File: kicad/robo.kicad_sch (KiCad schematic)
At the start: 46 parts, among them J10 KF2EDGR-2.54-2P, J11 KF7620-7.62-2P, J12 KF2EDGR-2.54-2P, J13 KF2EDGR-2.54-2P, J14 KF7620-7.62-2P, J15 PM254-2-12-Z-8.5, J16 PM254-2-09-Z-8.5, J8 KF2EDGR-2.54-4P, J9 KF2EDGR-2.54-3P, U16 74LVC1G17SE-7, U18 TPS70933DBVR, U19 74LVC1G17SE-7

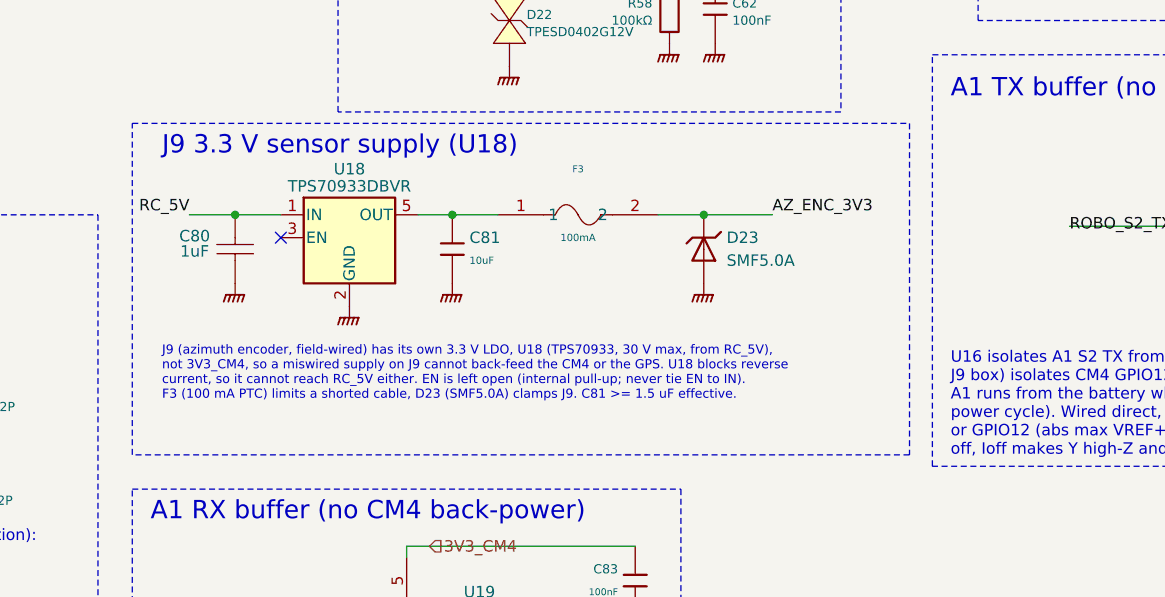
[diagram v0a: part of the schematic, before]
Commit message: Added notes
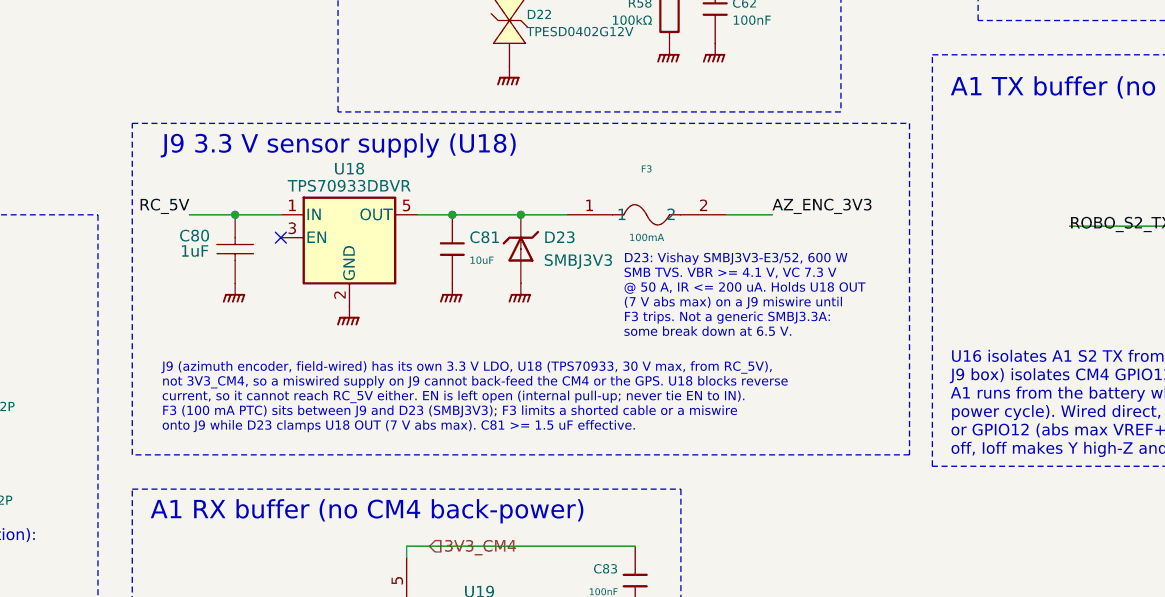
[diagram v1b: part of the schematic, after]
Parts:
- D23: value SMF5.0A -> SMBJ3V3; footprint MyPartsIPC:SODFL3718X110N -> MyPartsIPC:DIOM5436X244N; symbol MyParts:SMF5.0A -> MyParts:SMBJ3V3; LCSC Part C19077497 -> C82082; MPN SMF5.0A -> SMBJ3V3-E3/52; Manufacturer hongjiacheng -> Vishay; Pkg Type SMD SOD-123FL -> SMD SMB (DO-214AA)
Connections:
- net AZ_ENC_3V3: no longer D23.1
- net at C81.1, F3.1, U18.5 (OUT): now also D23.1
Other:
- note added: "D23: Vishay SMBJ3V3-E3/52, 600 W SMB TVS. VBR >= 4.1 V, VC 7.3 V @ 50 A, IR <= 200 uA. Holds U18 OUT (7 V abs max) on a J9 miswire until F3 trips. Not a generic SMBJ3.3A: some break down at 6.5 V."
- note added: "J9 (azimuth encoder, field-wired) has its own 3.3 V LDO, U18 (TPS70933, 30 V max, from RC_5V), not 3V3_CM4, so a miswired supply on J9 cannot back-feed the CM4 or the GPS. U18 blocks reverse current, so it cannot reach RC_5V either. EN is left open (internal pull-up; never tie EN to IN). F3 (100 mA PTC) sits between J9 and D23 (SMBJ3V3); F3 limits a shorted cable or a miswire onto J9 while D23 cl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"
- note removed: "J9 (azimuth encoder, field-wired) has its own 3.3 V LDO, U18 (TPS70933, 30 V max, from RC_5V), not 3V3_CM4, so a miswired supply on J9 cannot back-feed the CM4 or the GPS. U18 blocks reverse current, so it cannot reach RC_5V either. EN is left open (internal pull-up; never tie EN to IN). F3 (100 mA PTC) limits a shorted cable, D23 (SMF5.0A) clamps J9. C81 >= 1.5 uF effective."
- moved on the sheet: D23, F3
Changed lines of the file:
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@@
 		)
 	)
-	(text "J9 (azimuth encoder, field-wired) has its own 3.3 V LDO, U18 (TPS70933, 30 V max, from RC_5V),\nnot 3V3_CM4, so a miswired supply on J9 cannot back-feed the CM4 or the GPS. U18 blocks reverse\ncurrent, so it cannot reach RC_5V either. EN is left open (internal pull-up; never tie EN to IN).\nF3 (100 mA PTC) limits a shorted cable, D23 (SMF5.0A) clamps J9. C81 >= 1.5 uF effective."
+	(text "J9 (azimuth encoder, field-wired) has its own 3.3 V LDO, U18 (TPS70933, 30 V max, from RC_5V),\nnot 3V3_CM4, so a miswired supply on J9 cannot back-feed the CM4 or the GPS. U18 blocks reverse\ncurrent, so it cannot reach RC_5V either. EN is left open (internal pull-up; never tie EN to IN).\nF3 (100 mA PTC) sits between J9 and D23 (SMBJ3V3); F3 limits a shorted cable or a miswire\nonto J9 while D23 clamps U18 OUT (7 V abs max). C81 >= 1.5 uF effective."
 		(exclude_from_sim no)
-		(at 115.062 151.765 0)
+		(at 115.062 153.67 0)
 		(effects
 			(font
@@
 		)
 	)
+	(text "D23: Vishay SMBJ3V3-E3/52, 600 W\nSMB TVS. VBR >= 4.1 V, VC 7.3 V\n@ 50 A, IR <= 200 uA. Holds U18 OUT\n(7 V abs max) on a J9 miswire until\nF3 trips. Not a generic SMBJ3.3A:\nsome break down at 6.5 V."
+		(exclude_from_sim no)
+		(at 166.37 141.605 0)
+		(effects
+			(font
+				(size 1.016 1.016)
+			)
+			(justify left top)
+		)
+	)
 	(text "EMC: run motor leads in shielded cable, shield\nclamped 360 deg to the enclosure at the gland\n(not to J11/J14). Clip-on CM ferrite per pair at\nentry; 100 nF brush caps at the motors. Keep\nmotor leads away from GNSS/encoder wiring."
 		(exclude_from_sim no)
@@
 	)
 	(junction
-		(at 171.45 110.49)
+		(at 154.94 137.16)
 		(diameter 0)
 		(color 0 0 0 0)
 	)
 	(junction
-		(at 231.14 53.34)
+		(at 171.45 110.49)
 		(diameter 0)
 		(color 0 0 0 0)
 	)
 	(junction
-		(at 248.92 99.06)
+		(at 231.14 53.34)
 		(diameter 0)
 		(color 0 0 0 0)
 	)
 	(junction
-		(at 175.26 137.16)
+		(at 248.92 99.06)
 		(diameter 0)
 		(color 0 0 0 0)
@@
 	(wire
 		(pts
-			(xy 147.32 137.16) (xy 152.4 137.16)
+			(xy 147.32 137.16) (xy 160.02 137.16)
 		)
 		(stroke
@@
 	(wire
 		(pts
-			(xy 170.18 137.16) (xy 182.88 137.16)
+			(xy 177.8 137.16) (xy 182.88 137.16)
 		)
 		(stroke
@@
 	)
 	(symbol
-		(lib_id "MyParts:SMF5.0A")
-		(at 175.26 140.97 180)
+		(lib_id "MyParts:SMBJ3V3")
+		(at 154.94 140.97 180)
 		(unit 1)
 		(body_style 1)
@@
 		(dnp no)
 		(property "Reference" "D23"
-			(at 177.8 139.7 0)
+			(at 157.48 139.7 0)
 			(show_name no)
 			(do_not_autoplace no)
@@
 			)
 		)
-		(property "Value" "SMF5.0A"
-			(at 177.8 142.24 0)
+		(property "Value" "SMBJ3V3"
+			(at 157.48 142.24 0)
 			(show_name no)
 			(do_not_autoplace no)
@@
 			)
 		)
-		(property "Footprint" "MyPartsIPC:SODFL3718X110N"
-			(at 175.26 140.97 0)
+		(property "Footprint" "MyPartsIPC:DIOM5436X244N"
+			(at 154.94 140.97 0)
 			(hide yes)
 			(show_name no)
@@
 			)
 		)
-		(property "Datasheet" "${MYPARTS_DATASHEETS}/SMF5.0A.pdf"
-			(at 175.26 140.97 0)
+		(property "Datasheet" "${MYPARTS_DATASHEETS}/SMBJ3V3.pdf"
+			(at 154.94 140.97 0)
 			(hide yes)
 			(show_name no)
@@
 			)
 		)
-		(property "Description" "-55℃~+150℃ 1 200W@10/1000us 21.7A@10/1000us 400uA 5V 7V 9.2V IEC 61000-4-2 TVS Unidirectional SOD-123FL ESD and Surge Protection (TVS/ESD) ROHS"
-			(at 175.26 140.97 0)
+		(property "Description" "-55℃~+175℃ 1 600W@10/1000us 50A@10/1000us 200uA 3.3V 4.1V 7.3V TVS Unidirectional SMB(DO-214AA) ESD and Surge Protection (TVS/ESD) ROHS"
+			(at 154.94 140.97 0)
 			(hide yes)
 			(show_name no)
@@
 			)
 		)
-		(property "Manufacturer" "hongjiacheng"
-			(at 175.26 140.97 0)
+		(property "Manufacturer" "Vishay"
+			(at 154.94 140.97 0)
 			(hide yes)
 			(show_name no)
@@
 		)
 		(property "ki_keywords" ""
-			(at 175.26 140.97 0)
+			(at 154.94 140.97 0)
 			(hide yes)
 			(show_name no)
@@
 		)
 		(property "ki_fp_filters" "D_*"
-			(at 175.26 140.97 0)
+			(at 154.94 140.97 0)
 			(hide yes)
 			(show_name no)
@@
 			)
 		)
-		(property "MPN" "SMF5.0A"
-			(at 175.26 140.97 0)
+		(property "MPN" "SMBJ3V3-E3/52"
+			(at 154.94 140.97 0)
 			(hide yes)
 			(show_name no)
@@
 			)
 		)
-		(property "LCSC Part" "C19077497"
-			(at 175.26 140.97 0)
+		(property "LCSC Part" "C82082"
+			(at 154.94 140.97 0)
 			(hide yes)
 			(show_name no)
@@
 			)
 		)
-		(property "Pkg Type" "SMD SOD-123FL"
-			(at 175.26 140.97 0)
+		(property "Pkg Type" "SMD SMB (DO-214AA)"
+			(at 154.94 140.97 0)
 			(hide yes)
 			(show_name no)
@@
 	(symbol
 		(lib_id "MyParts:nSMD010")
-		(at 161.29 135.89 0)
+		(at 168.91 135.89 0)
 		(unit 1)
 		(body_style 1)
@@
 		(dnp no)
 		(property "Reference" "F3"
-			(at 161.29 132.08 0)
+			(at 168.91 132.08 0)
 			(show_name no)
 			(do_not_autoplace no)
@@
 		)
 		(property "Value" "100mA"
-			(at 161.29 139.7 0)
+			(at 168.91 139.7 0)
 			(show_name no)
 			(do_not_autoplace yes)
@@
 		)
 		(property "Footprint" "MyPartsIPC:FUSC3216X110N"
-			(at 161.29 135.89 0)
+			(at 168.91 135.89 0)
 			(hide yes)
 			(show_name no)
@@
 		)
 		(property "Datasheet" "${MYPARTS_DATASHEETS}/nSMD010.pdf"
-			(at 161.29 135.89 0)
+			(at 168.91 135.89 0)
 			(hide yes)
 			(show_name no)
@@
 		)
 		(property "Description" "PTC resettable fuse 100mA hold 250mA trip 60V 1206, 1.6 ohm initial"
-			(at 161.29 135.89 0)
+			(at 168.91 135.89 0)
 			(hide yes)
 			(show_name no)
@@
 		)
 		(property "Manufacturer" "TECHFUSE"
-			(at 161.29 135.89 0)
+			(at 168.91 135.89 0)
 			(hide yes)
 			(show_name no)
@@
 		)
 		(property "MPN" "nSMD010"
-			(at 161.29 135.89 0)
+			(at 168.91 135.89 0)
 			(hide yes)
 			(show_name no)
@@
 		)
 		(property "LCSC Part" "C70065"
-			(at 161.29 135.89 0)
+			(at 168.91 135.89 0)
 			(hide yes)
 			(show_name no)
@@
 		)
 		(property "Pkg Type" "SMD 1206"
-			(at 161.29 135.89 0)
+			(at 168.91 135.89 0)
 			(hide yes)
 			(show_name no)
@@
 	(symbol
 		(lib_id "power:GNDPWR")
-		(at 175.26 144.78 0)
+		(at 154.94 144.78 0)
 		(unit 1)
 		(body_style 1)
@@
 		(dnp no)
 		(property "Reference" "#PWR0456"
-			(at 175.26 151.13 0)
+			(at 154.94 151.13 0)
 			(hide yes)
 			(show_name no)
@@
 		)
 		(property "Value" "PGND"
-			(at 175.26 148.59 0)
+			(at 154.94 148.59 0)
 			(hide yes)
 			(show_name no)
@@
 		)
 		(property "Footprint" ""
-			(at 175.26 144.78 0)
+			(at 154.94 144.78 0)
 			(hide yes)
 			(show_name no)
@@
 		)
 		(property "Datasheet" ""
-			(at 175.26 144.78 0)
+			(at 154.94 144.78 0)
 			(hide yes)
 			(show_name no)
@@
 		)
 		(property "Description" "Power symbol creates a global label with name \"GNDPWR\" , global ground"
-			(at 175.26 144.78 0)
+			(at 154.94 144.78 0)
 			(hide yes)
 			(show_name no)
